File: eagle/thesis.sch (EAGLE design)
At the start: 18 parts, among them J1 RJ11-6PTH, U1 ITG-3200, U2 ADXL362

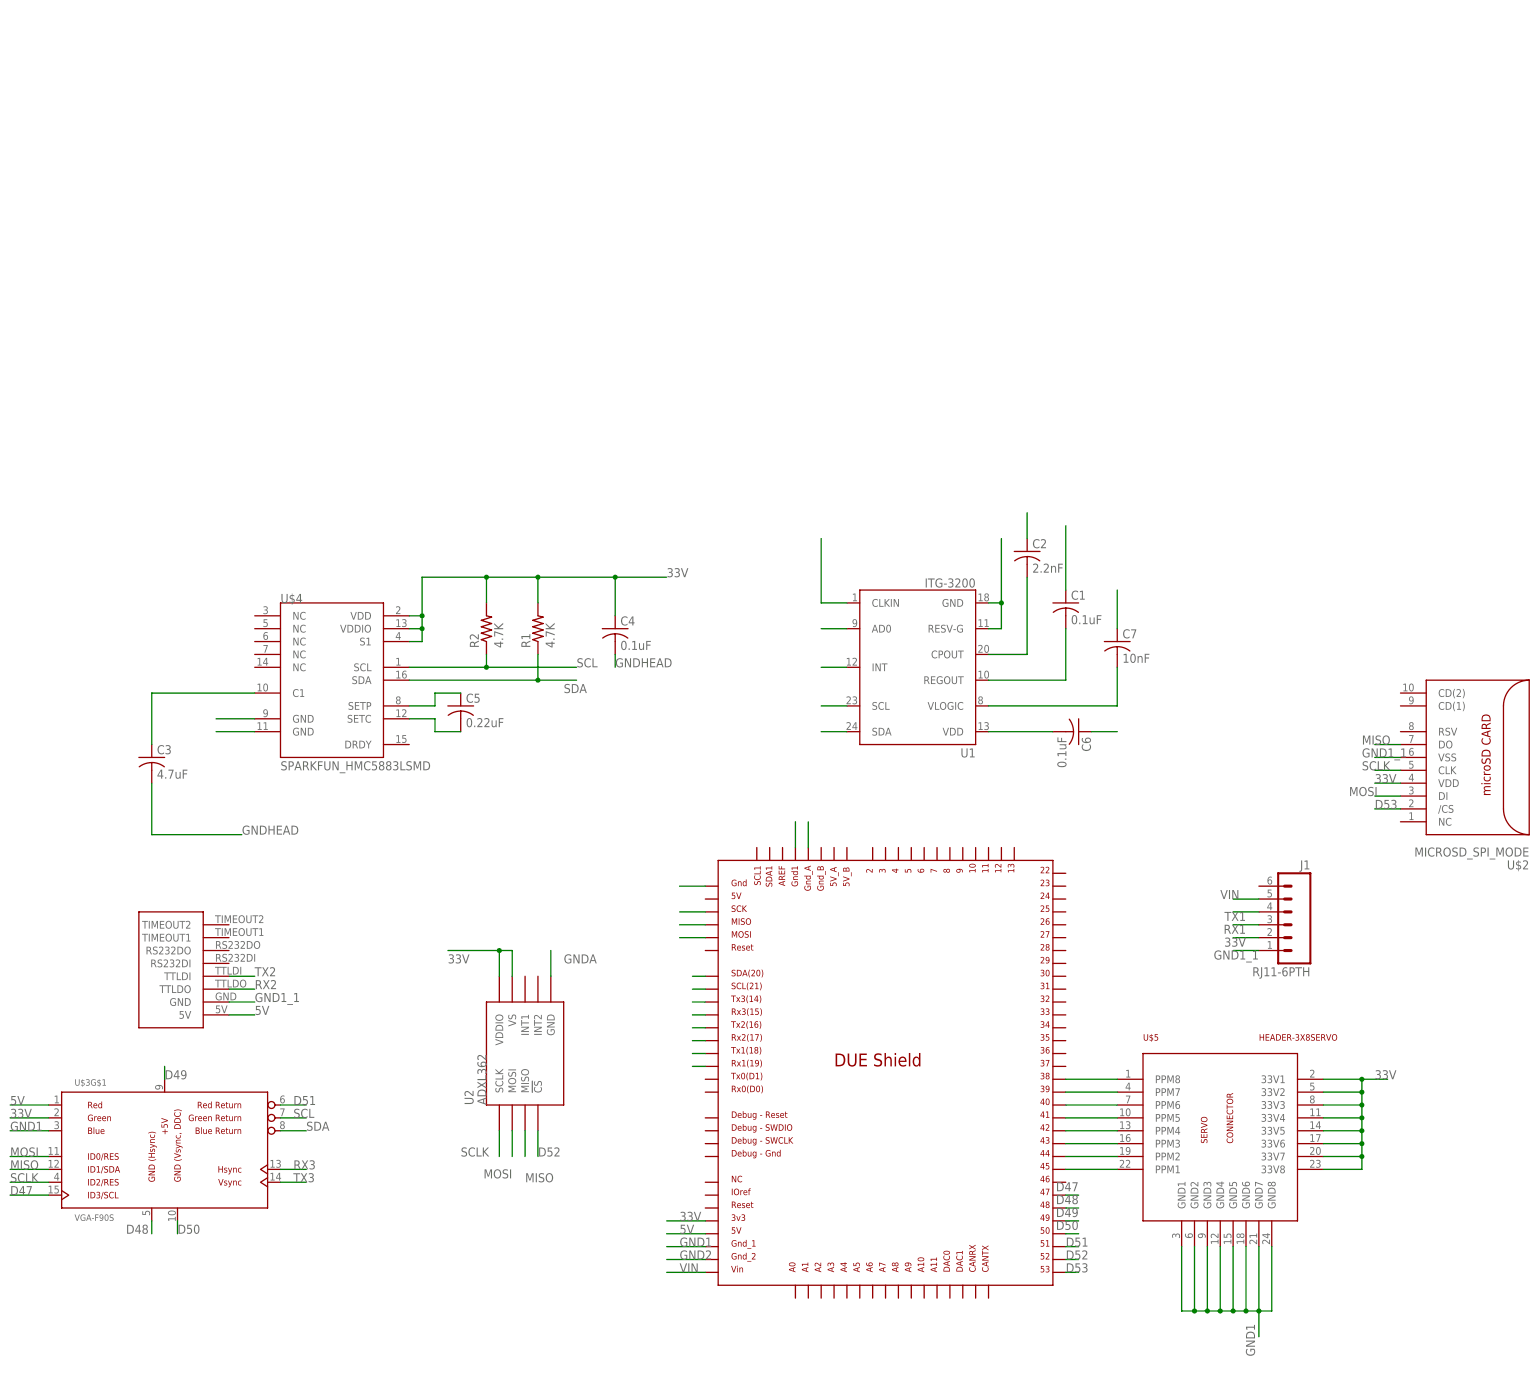
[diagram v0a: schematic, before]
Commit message: wrote a bunch and added references and pictures
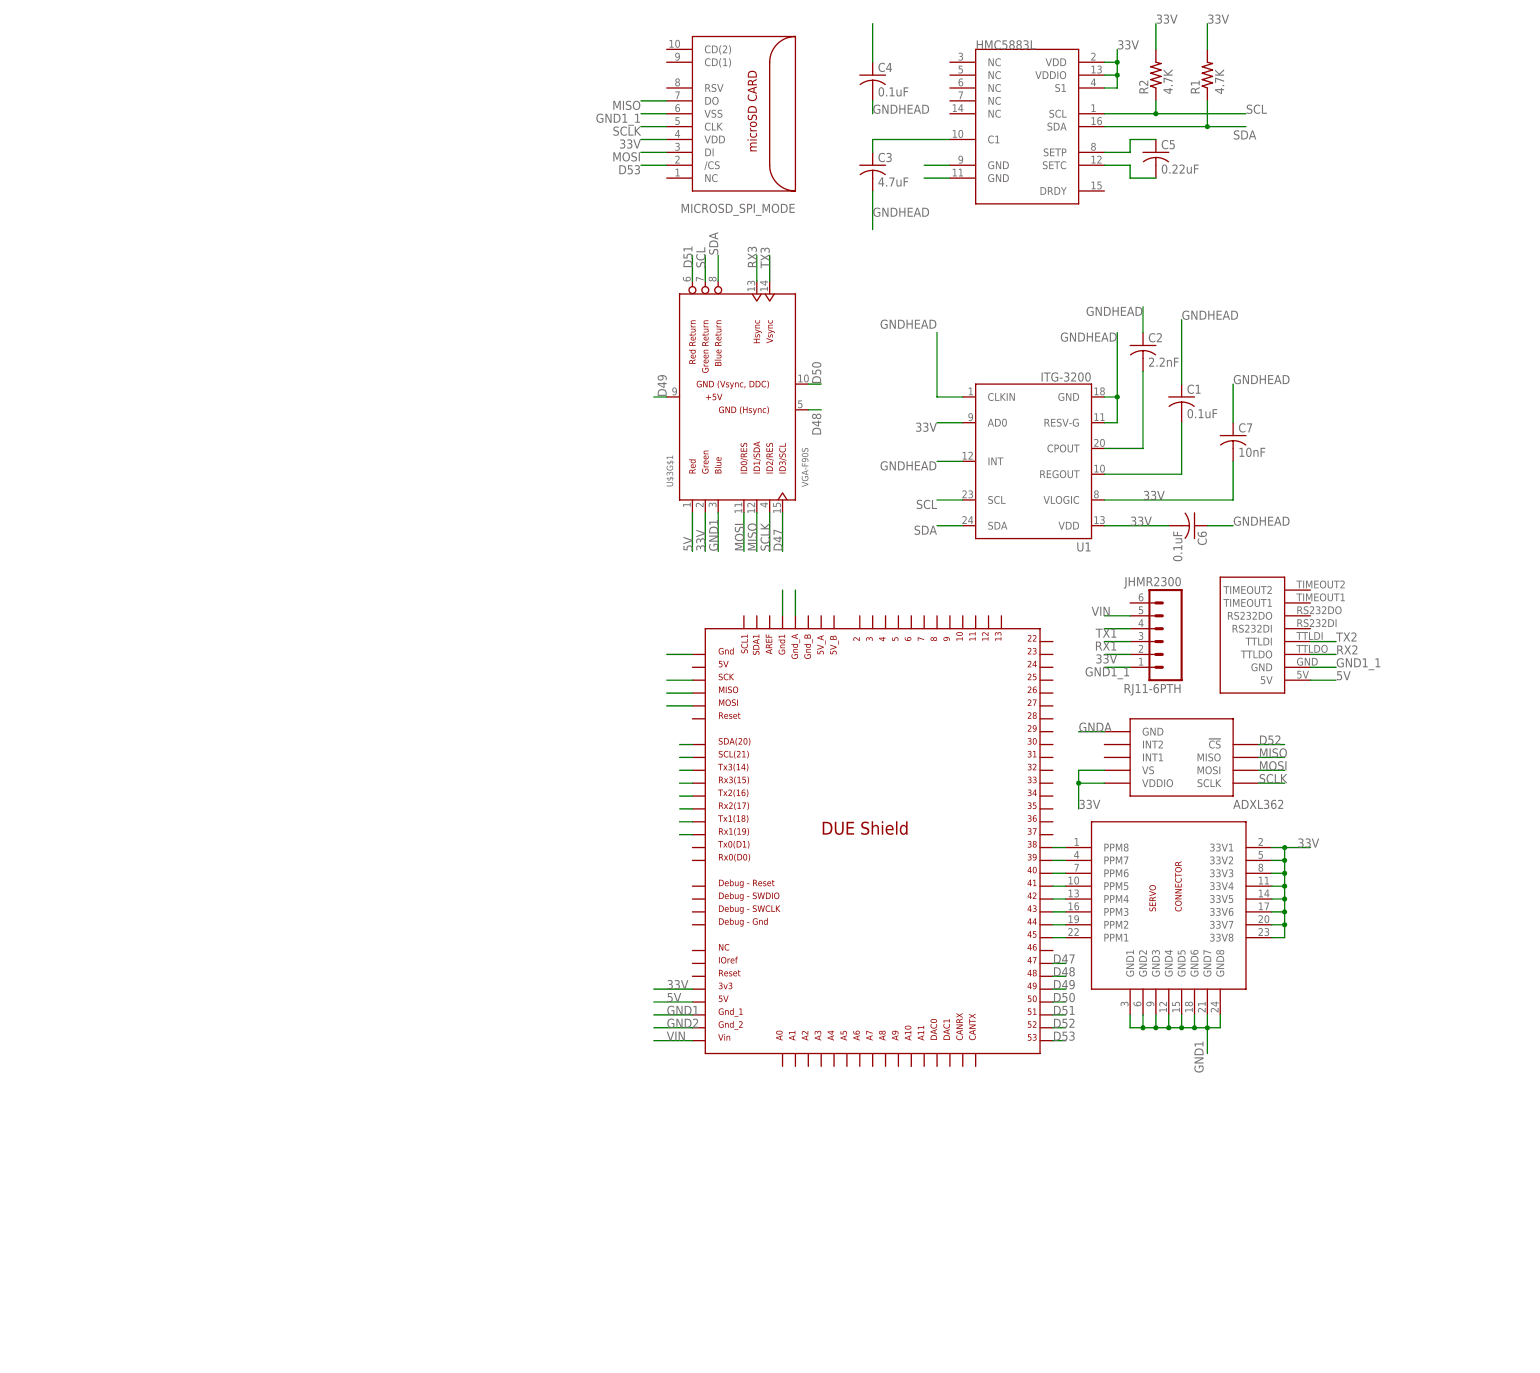
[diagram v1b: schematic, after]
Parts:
- removed J1: RJ11-6PTH, SparkFun-Connectors:RJ11-6PTH
- removed U$4: SPARKFUN_HMC5883LSMD, HMC5883L_Breakout-v11:SPARKFUN_HMC5883LSMD
- added HMC5883L: SPARKFUN_HMC5883LSMD, HMC5883L_Breakout-v11:SPARKFUN_HMC5883LSMD
- added JHMR2300: RJ11-6PTH, SparkFun-Connectors:RJ11-6PTH
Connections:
- net 33V: now also C6.2, HMC5883L.S1, HMC5883L.VDD, HMC5883L.VDDIO, JHMR2300.2; no longer J1.2, U$4.S1, U$4.VDD, U$4.VDDIO
- net GND1_1: now also JHMR2300.1; no longer J1.1
- net GNDHEAD: now also HMC5883L.GND@1, HMC5883L.GND@2; no longer U$4.GND@1, U$4.GND@2
- net N$12: now also HMC5883L.C1; no longer U$4.C1
- net N$5: now also HMC5883L.SETP; no longer U$4.SETP
- net N$7: now also HMC5883L.SETC; no longer U$4.SETC
- net RX1: now also JHMR2300.3; no longer J1.3
- net SCL: now also HMC5883L.SCL; no longer U$4.SCL
- net SDA: now also HMC5883L.SDA; no longer U$4.SDA
- net TX1: now also JHMR2300.4; no longer J1.4
- net VIN: now also JHMR2300.5; no longer J1.5
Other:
- moved on the sheet: C1, C2, C3, C4, C5, C6, C7, R1, R2, U$3G$1, U1
